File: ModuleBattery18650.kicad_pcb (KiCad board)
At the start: 2 copper layers, 100 x 30 mm, 26 parts, among them J1 Connector_2p, J2 Connector_2p_r, T1 SISH615ADN, T2 SISH615ADN, T3 FDN337N, T4 SISH615ADN, T5 SISH615ADN, U1 MCP121T-315E

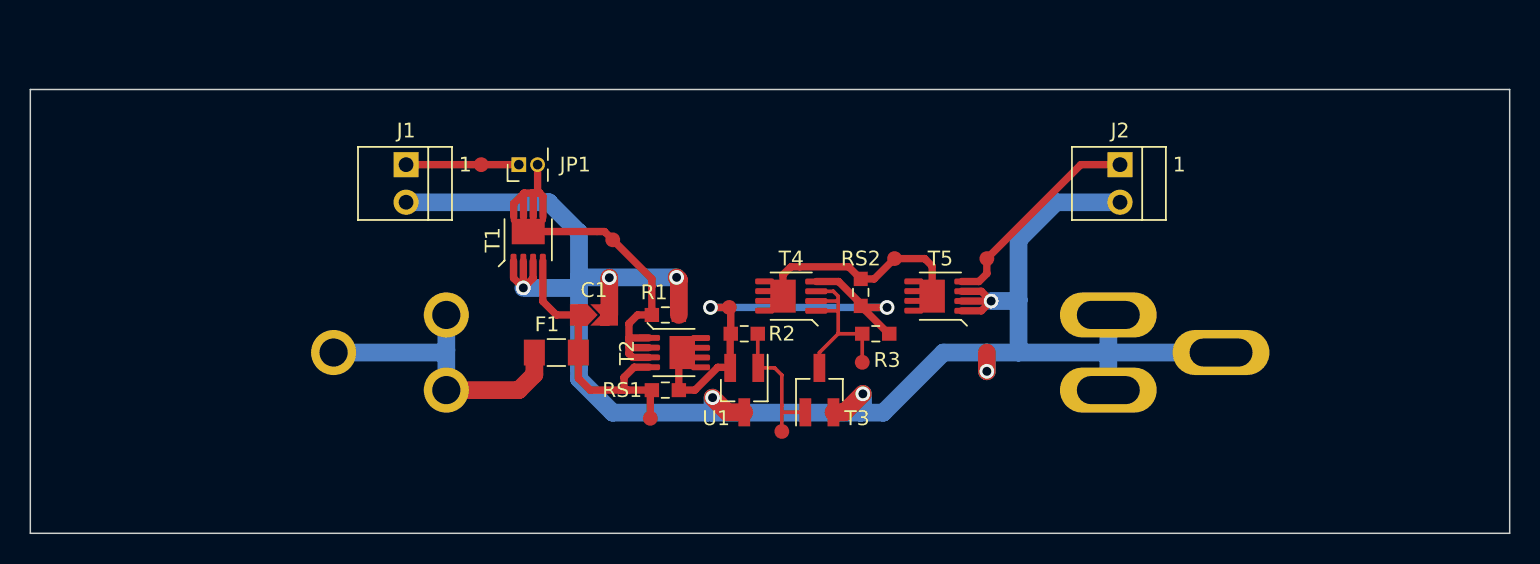
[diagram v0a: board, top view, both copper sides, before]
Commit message: rev00
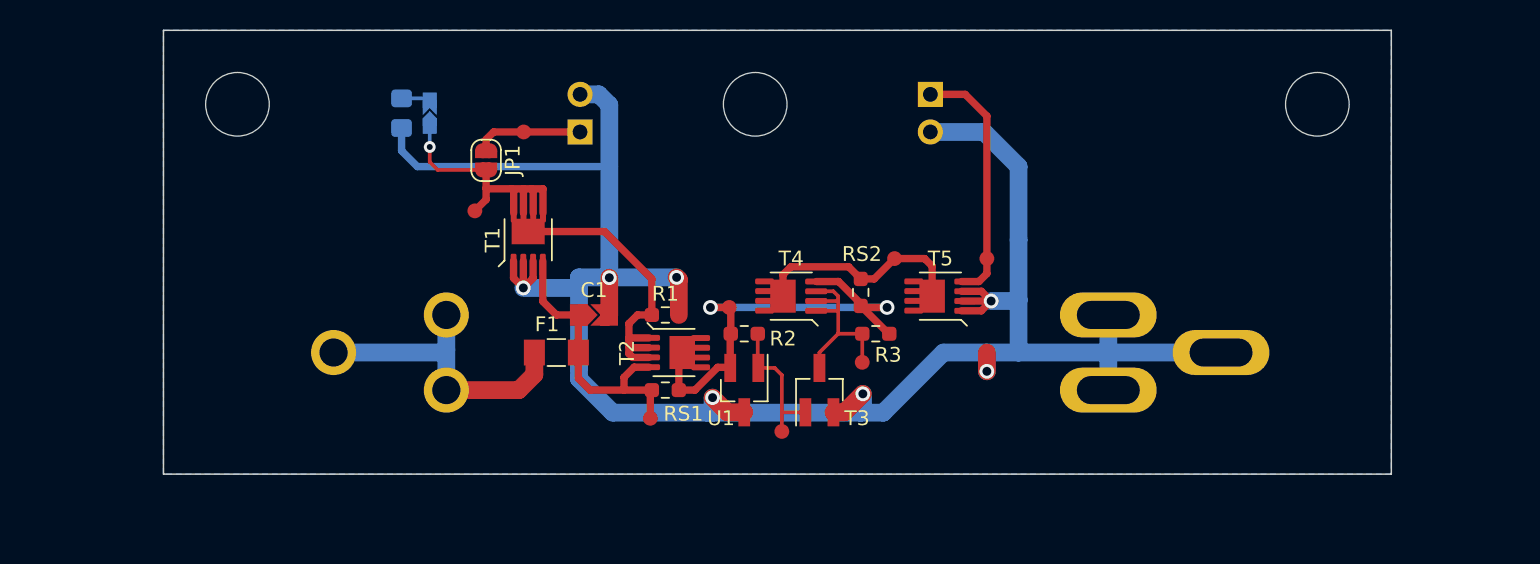
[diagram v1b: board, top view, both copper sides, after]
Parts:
- added D1: LED, 0ESN_Lib:D_0603_1608Metric_Pad1.05x0.95mm_HandSolder, B.Cu at (127.0, 101.6)
- added R4: 150R, Resistor_SMD:R_0805_2012Metric_Pad1.20x1.40mm_HandSolder, B.Cu at (125.1, 101.6)
- added REF**: MountingHole_4.3mm_M4, MountingHole:MountingHole_4.3mm_M4, F.Cu at (114.0, 101.0)
- added REF**: MountingHole_4.3mm_M4, MountingHole:MountingHole_4.3mm_M4, F.Cu at (187.0, 101.0)
- added REF**: MountingHole_4.3mm_M4, MountingHole:MountingHole_4.3mm_M4, F.Cu at (149.0, 101.0)
- J1, J2: moved to B.Cu
- JP1: footprint 0ESN_Lib:PinHeader_1x02_P1.27mm_Vertical -> Jumper:SolderJumper-2_P1.3mm_Open_RoundedPad1.0x1.5mm
- R1, R2, R3, RS1, RS2: footprint 0ESN_Lib:R_0603_1608Metric_Pad0.98x0.95mm_HandSolder -> Resistor_SMD:R_0603_1608Metric_Pad0.98x0.95mm_HandSolder
- moved J2 13.7 mm to (160.8, 100.3), turned to 180 degrees
- moved J1 12.0 mm to (137.2, 102.9)
- moved TP3 9.52 mm to (130.0, 108.2)
- moved TP1 3.62 mm to (133.3, 102.9)
- moved JP1 2.23 mm to (130.8, 104.8), turned to -90 degrees
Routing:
- net GND: track 129.0 -> 147.4 mm
- net Net-(JP1-Pad2): track 30.1 -> 40.2 mm, vias 0 -> 1
- net /Vbat: track 14.6 -> 17.0 mm
- net Net-(D1-Pad2): track 0.00 -> 1.96 mm
- added copper zone on B.Cu, net GND
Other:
- board size 100 x 30 mm -> 83 x 30 mm
- board text added: "CHARGE"
- board text added: "ModuleBattery18650 Nicolas Esseiva 2023.04.08 - r00"
- board text added: "POWER"
